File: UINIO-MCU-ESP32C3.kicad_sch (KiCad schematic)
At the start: 41 parts, among them J1 Conn_01x15_Male, J2 外接串行下载接口, J3 Conn_01x15_Male, SW1 复位按键, SW2 下载按键, U1 ME6211C33M5G-N, U2 W25Q128JVSSIQ, U3 ESP32-C3, U4 CH343P, Y1 40MHz

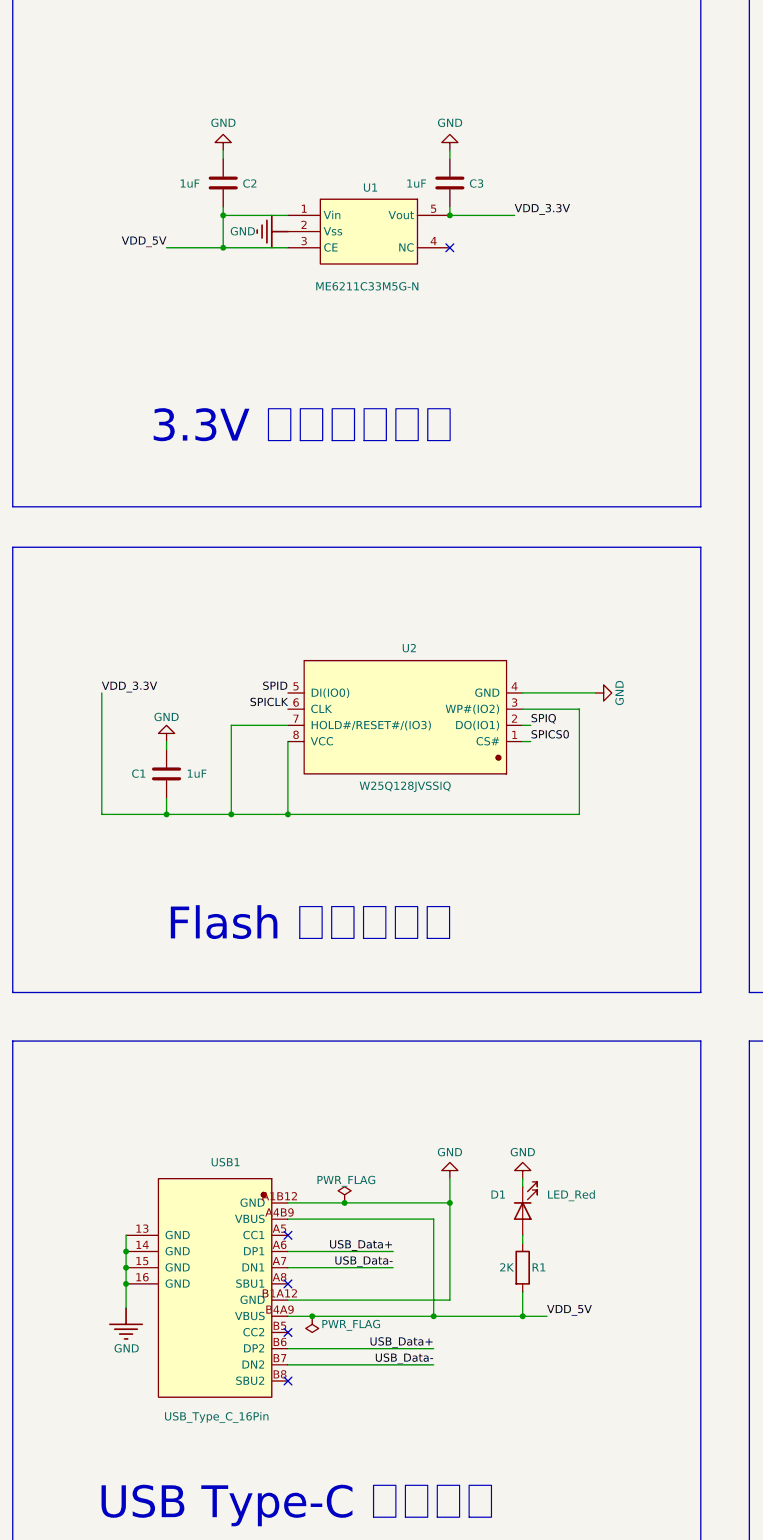
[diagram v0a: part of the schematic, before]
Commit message: Prepare version 3.0.0.
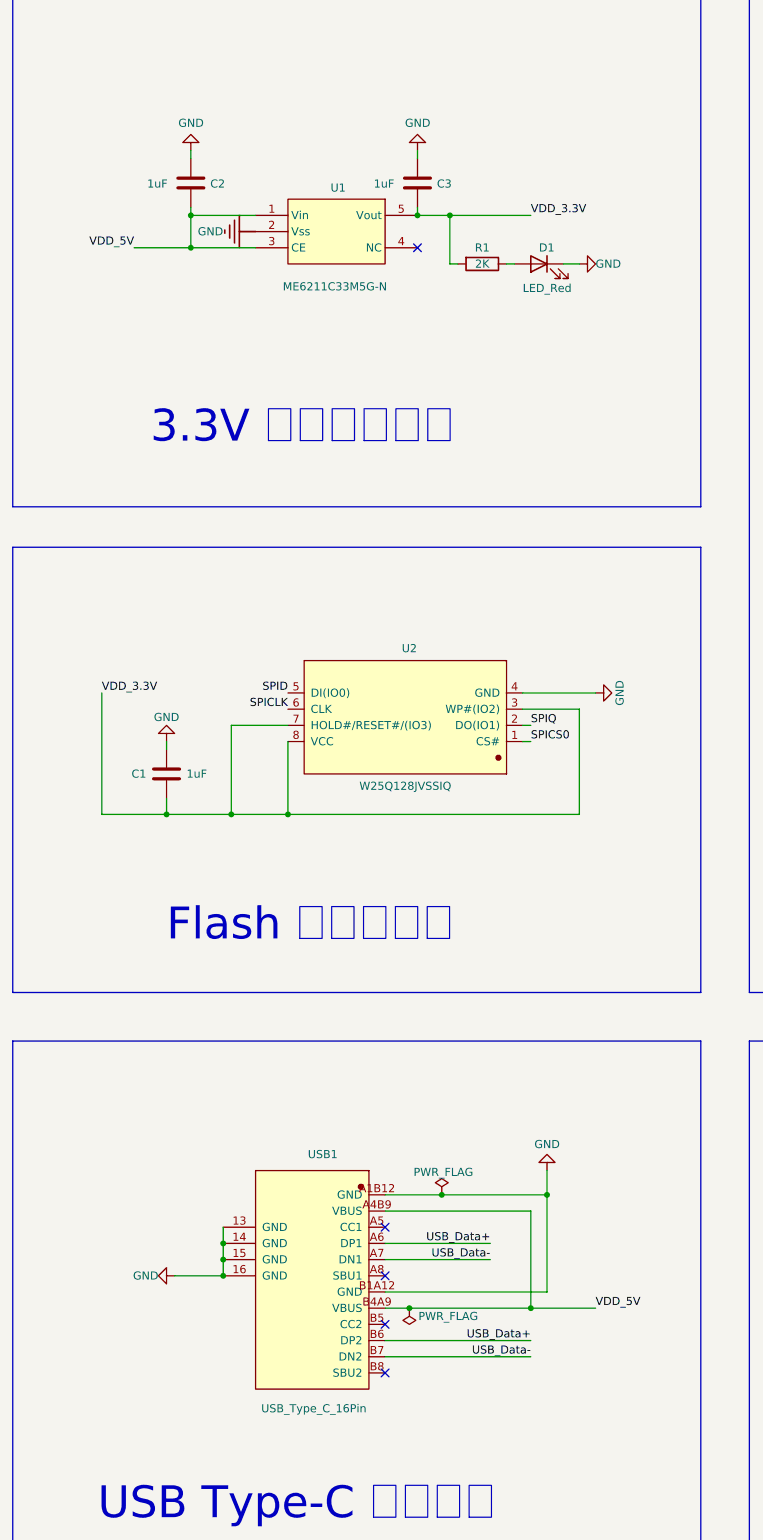
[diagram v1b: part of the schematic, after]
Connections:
- net VDD_3.3V: now also R1.2
- net VDD_5V: no longer R1.2
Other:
- moved on the sheet: C2, C3, D1, R1, U1, USB1
